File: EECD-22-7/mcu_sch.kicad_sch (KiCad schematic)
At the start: 1 part

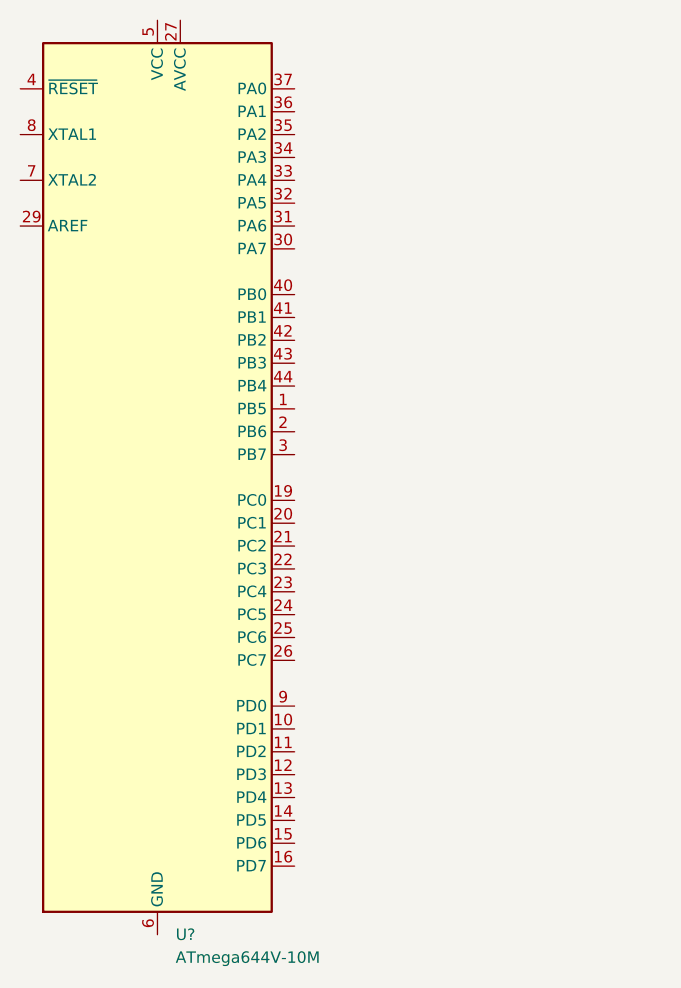
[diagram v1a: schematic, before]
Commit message: Add files via upload
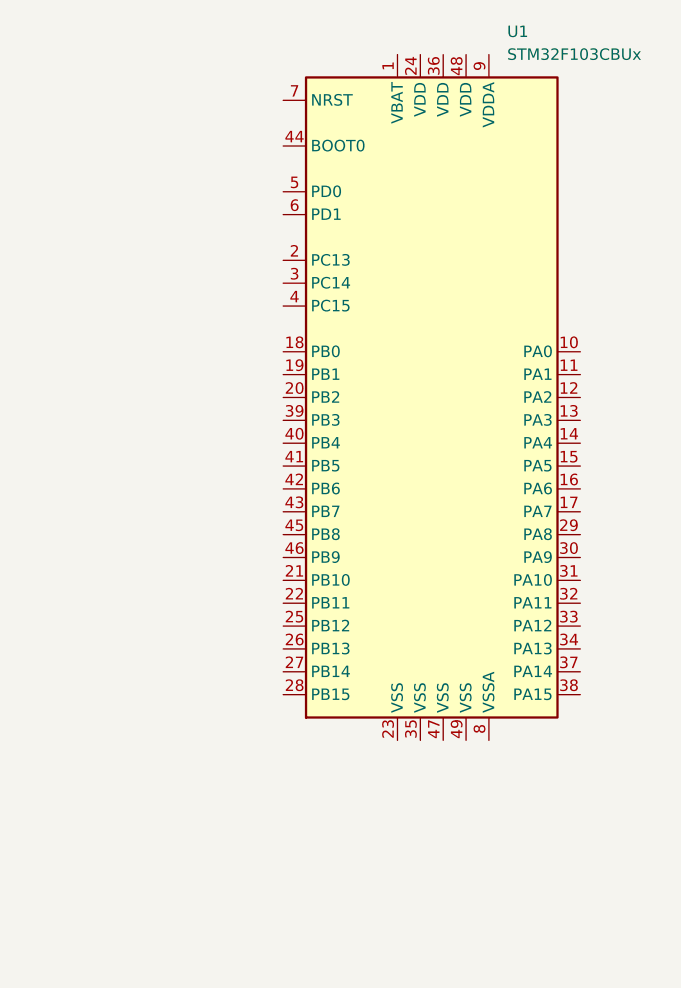
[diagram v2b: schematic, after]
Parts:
- removed U?: ATmega644V-10M, Package_DFN_QFN:QFN-44-1EP_7x7mm_P0.5mm_EP5.2x5.2mm, symbol MCU_Microchip_ATmega:ATmega644V-10M
- added U1: STM32F103CBUx, Package_DFN_QFN:QFN-48-1EP_7x7mm_P0.5mm_EP5.6x5.6mm, symbol MCU_ST_STM32F1:STM32F103CBUx
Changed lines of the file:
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@@
 (kicad_sch (version 20211123) (generator eeschema)
   (paper "A4")
-  (symbol (lib_id "MCU_Microchip_ATmega:ATmega644V-10M") (at 120.65 91.44 0) (unit 1)
+  (symbol (lib_id "MCU_ST_STM32F1:STM32F103CBUx") (at 152.4 82.55 0) (unit 1)
     (in_bom yes) (on_board yes) (fields_autoplaced)
-    (property "Reference" "U?" (id 0) (at 122.6694 142.24 0)
+    (property "Reference" "U1" (id 0) (at 159.4994 41.91 0)
       (effects (font (size 1.27 1.27)) (justify left))
     )
-    (property "Value" "ATmega644V-10M" (id 1) (at 122.6694 144.78 0)
+    (property "Value" "STM32F103CBUx" (id 1) (at 159.4994 44.45 0)
       (effects (font (size 1.27 1.27)) (justify left))
     )
-    (property "Footprint" "Package_DFN_QFN:QFN-44-1EP_7x7mm_P0.5mm_EP5.2x5.2mm" (id 2) (at 120.65 91.44 0)
-      (effects (font (size 1.27 1.27) italic) hide)
+    (property "Footprint" "Package_DFN_QFN:QFN-48-1EP_7x7mm_P0.5mm_EP5.6x5.6mm" (id 2) (at 137.16 118.11 0)
+      (effects (font (size 1.27 1.27)) (justify right) hide)
     )
-    (property "Datasheet" "http://ww1.microchip.com/downloads/en/DeviceDoc/doc2593.pdf" (id 3) (at 120.65 91.44 0)
+    (property "Datasheet" "http://www.st.com/st-web-ui/static/active/en/resource/technical/document/datasheet/CD00161566.pdf" (id 3) (at 152.4 82.55 0)
       (effects (font (size 1.27 1.27)) hide)
     )
@@
     (pin "44")
     (pin "45")
+    (pin "46")
+    (pin "47")
+    (pin "48")
+    (pin "49")
     (pin "5")
     (pin "6")

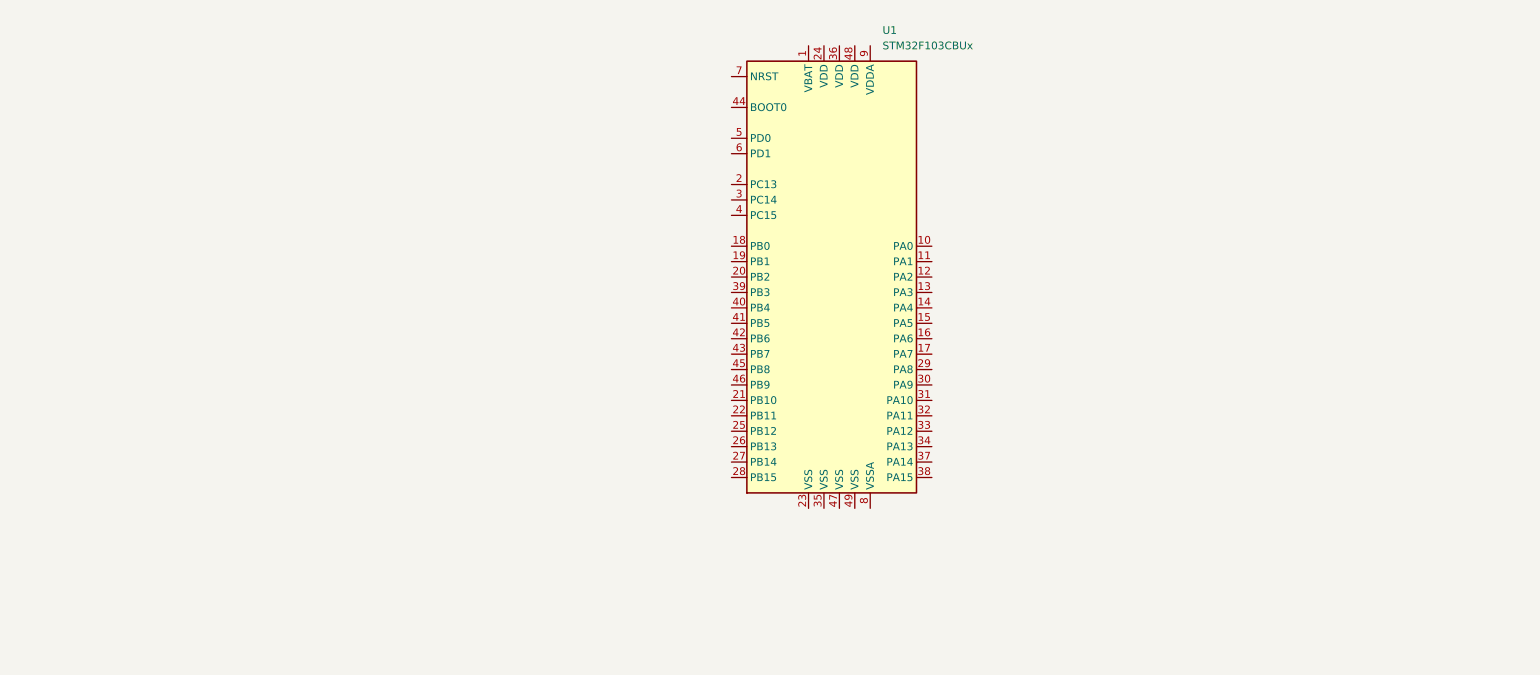
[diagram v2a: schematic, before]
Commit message: Add files via upload
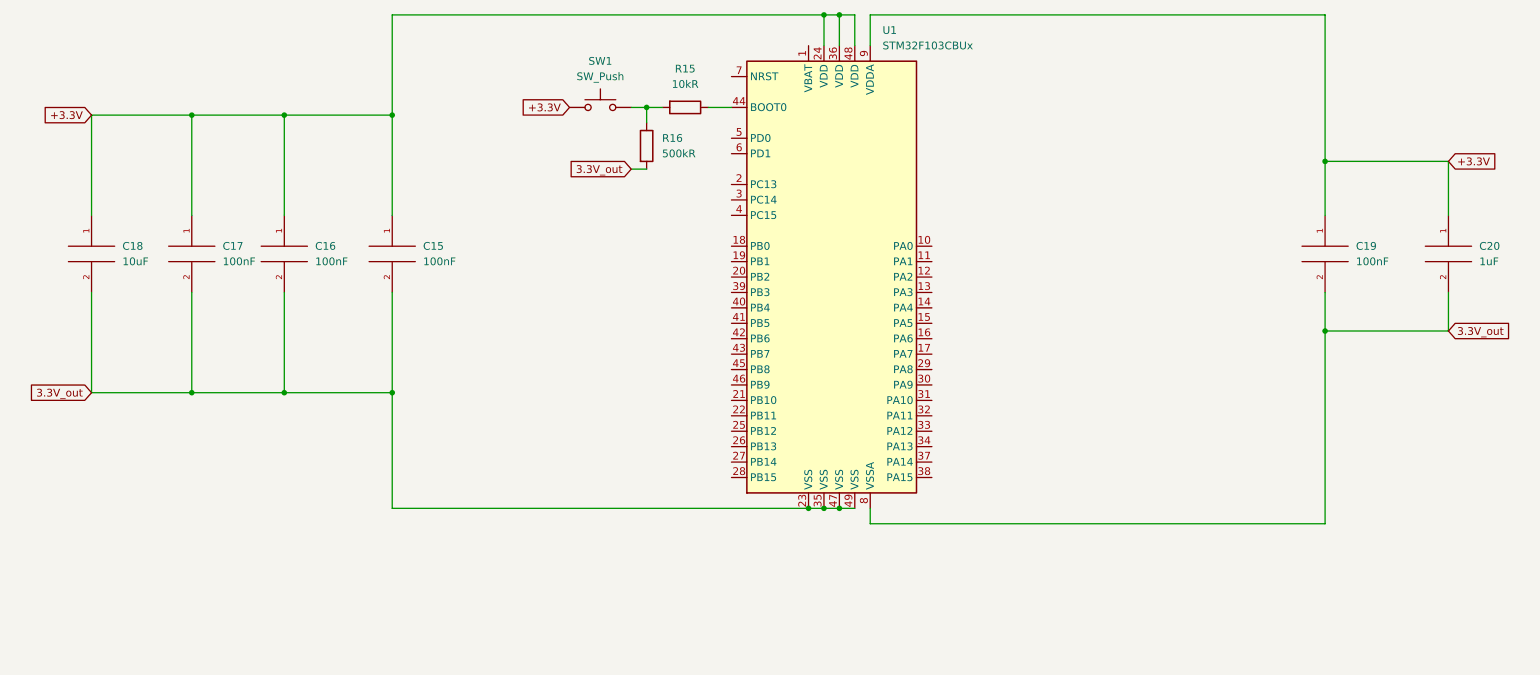
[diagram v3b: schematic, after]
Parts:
- added C15, C16, C17, C19: 100nF, symbol pspice:C
- added C18: 10uF, symbol pspice:C
- added C20: 1uF, symbol pspice:C
- added R15: 10kR, symbol Device:R
- added R16: 500kR, symbol Device:R
- added SW1: SW_Push, symbol Switch:SW_Push
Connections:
- net 3.3V_out: now reaches U1.23 (VSS)
- net 3.3V_out: now also U1.35 (VSS), U1.47 (VSS), U1.49 (VSS), U1.8 (VSSA), C15.2, C16.2, C17.2, C18.2, C19.2, C20.2, R16.2
- net +3.3V: now reaches U1.24 (VDD)
- net +3.3V: now also U1.36 (VDD), U1.48 (VDD), U1.9 (VDDA), C15.1, C16.1, C17.1, C18.1, C19.1, C20.1, SW1.1
- net at U1.44 (BOOT0): now also R15.1
- new net: R15.2, R16.1, SW1.2
